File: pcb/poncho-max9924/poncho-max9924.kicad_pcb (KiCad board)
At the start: 2 copper layers, 48 parts, among them J1 Screw_Terminal_01x02, J2 Screw_Terminal_01x02, J3 jumper_4_open, U1 MAX9924, U2 MAX9000

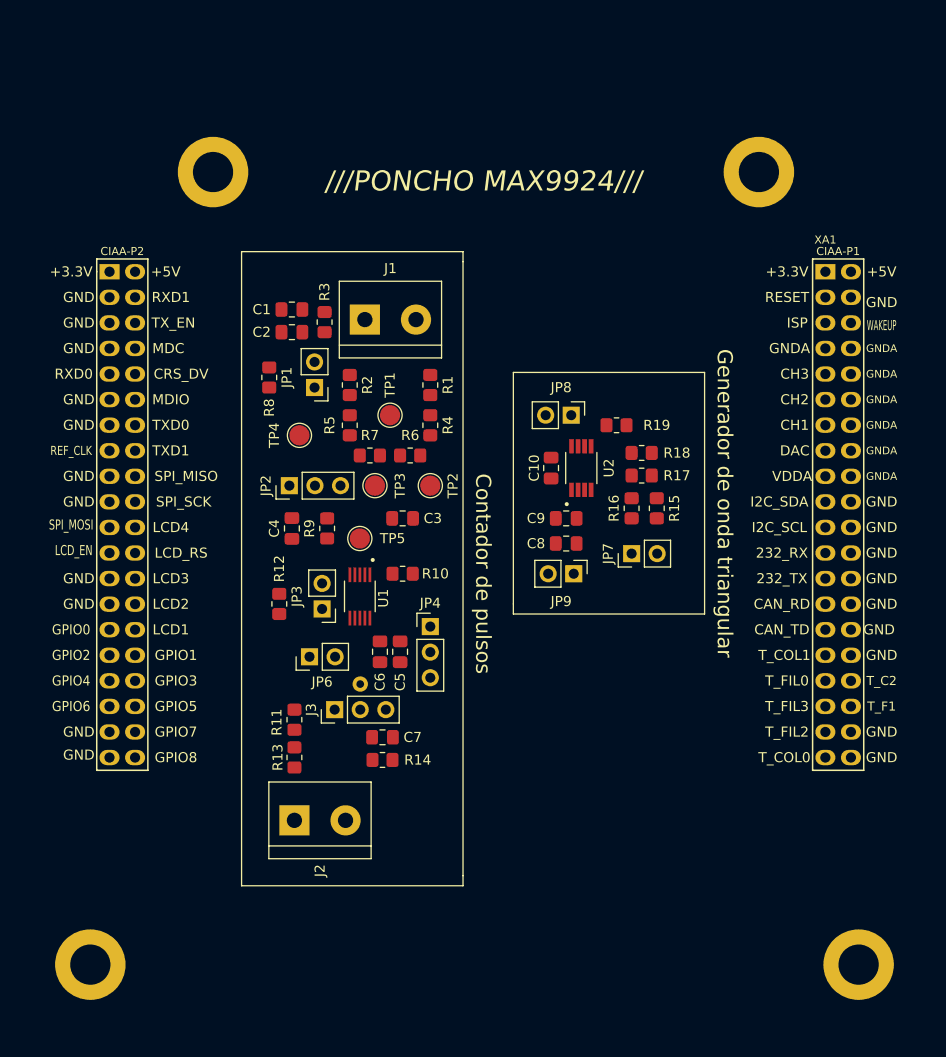
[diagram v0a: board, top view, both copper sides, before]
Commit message: primer routeado
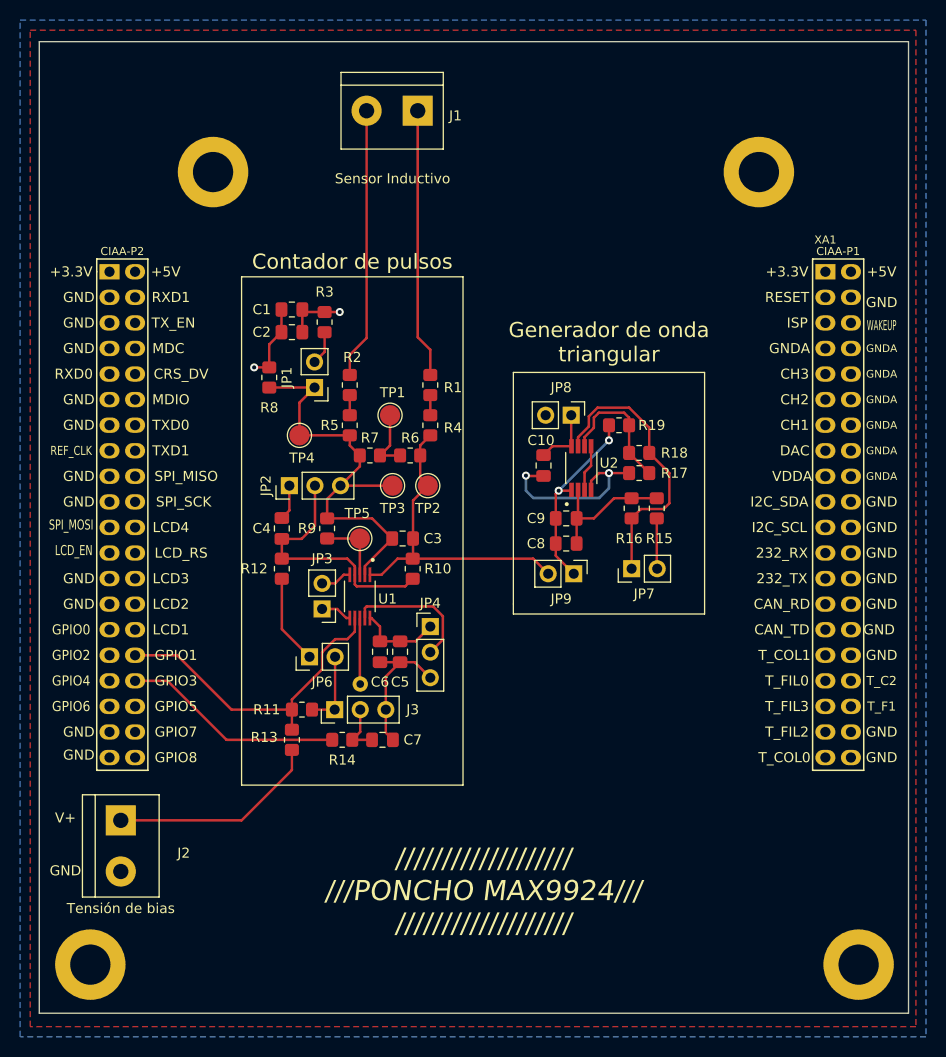
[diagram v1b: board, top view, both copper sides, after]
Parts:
- moved J1 21.4 mm to (144.5, 53.0), turned to 180 degrees
- moved J2 17.2 mm to (115.0, 123.5), turned to 270 degrees
- moved R14 4.47 mm to (137.0, 115.5), turned to 0 degrees
- moved R12 3.51 mm to (131.0, 98.5)
- moved C3 2.00 mm to (143.0, 95.5)
- moved R13 1.77 mm to (132.0, 115.5)
- moved TP3 1.75 mm to (142.0, 90.2)
- moved JP7 1.50 mm to (165.8, 98.5)
- moved R11 1.25 mm to (133.0, 112.5), turned to 0 degrees
- moved R10 1.12 mm to (144.0, 98.5), turned to 90 degrees
- moved C4 1.00 mm to (131.0, 94.5), turned to 90 degrees
- moved C10 0.79 mm to (157.0, 88.2)
- moved R17 0.35 mm to (166.5, 89.0)
- moved C7 0.25 mm to (141.0, 115.5)
- moved R18 0.25 mm to (166.5, 87.0), turned to 180 degrees
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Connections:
- R1 pad 2: Net-(J1-Pad2) -> Net-(J1-Pad1)
- R2 pad 2: Net-(J1-Pad1) -> Net-(J1-Pad2)
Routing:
- net GND: track 0.00 -> 47.3 mm, vias 0 -> 3
- net Net-(C3-Pad2): track 0.00 -> 42.1 mm
- net /AOUT: track 0.00 -> 32.6 mm
- net /COUT: track 0.00 -> 32.2 mm
- net /COUT_2: track 0.00 -> 28.3 mm
- net Net-(J1-Pad2): track 0.00 -> 26.9 mm
- net Net-(J1-Pad1): track 0.00 -> 26.8 mm
- net /BIAS: track 0.00 -> 25.3 mm
- net /FILTER: track 0.00 -> 22.0 mm
- net /V_PULL: track 0.00 -> 21.1 mm
- net Net-(C8-Pad2): track 0.00 -> 19.0 mm, vias 0 -> 2
- net +5V: track 0.00 -> 14.8 mm, vias 0 -> 1
- net Net-(C8-Pad1): track 0.00 -> 14.2 mm
- net Net-(R17-Pad1): track 0.00 -> 14.0 mm
- net Net-(JP4-Pad2): track 0.00 -> 13.3 mm
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- added copper zone on B.Cu, net +5V
- added copper zone on F.Cu, net GND
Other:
- board outline added: 86.4 x 96.5 mm
- board text added: "/////////////////// ///PONCHO MAX9924/// ///////////////////"
- board text added: "GND"
- board text added: "Material: FR4 Espesor: 1.6mm Componentes: Solo lado top. Serigrafia: Solo lado top, color: blanco. Grillas: 0.25mm, 0.5mm, 1mm"
- board text added: "Sensor Inductivo"
- board text added: "Tensión de bias"
- board text added: "V+"
- board text removed: "///PONCHO MAX9924///"
